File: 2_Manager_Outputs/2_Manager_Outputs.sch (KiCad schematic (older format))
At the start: 17 parts, among them J11 I2C, J2 RS232, P2 CONN_01X04, P3 SPI, P4 CONN_01X04, U1 ATMEGA328P-AU_MIO, U4 LD1117S33TR_MIO

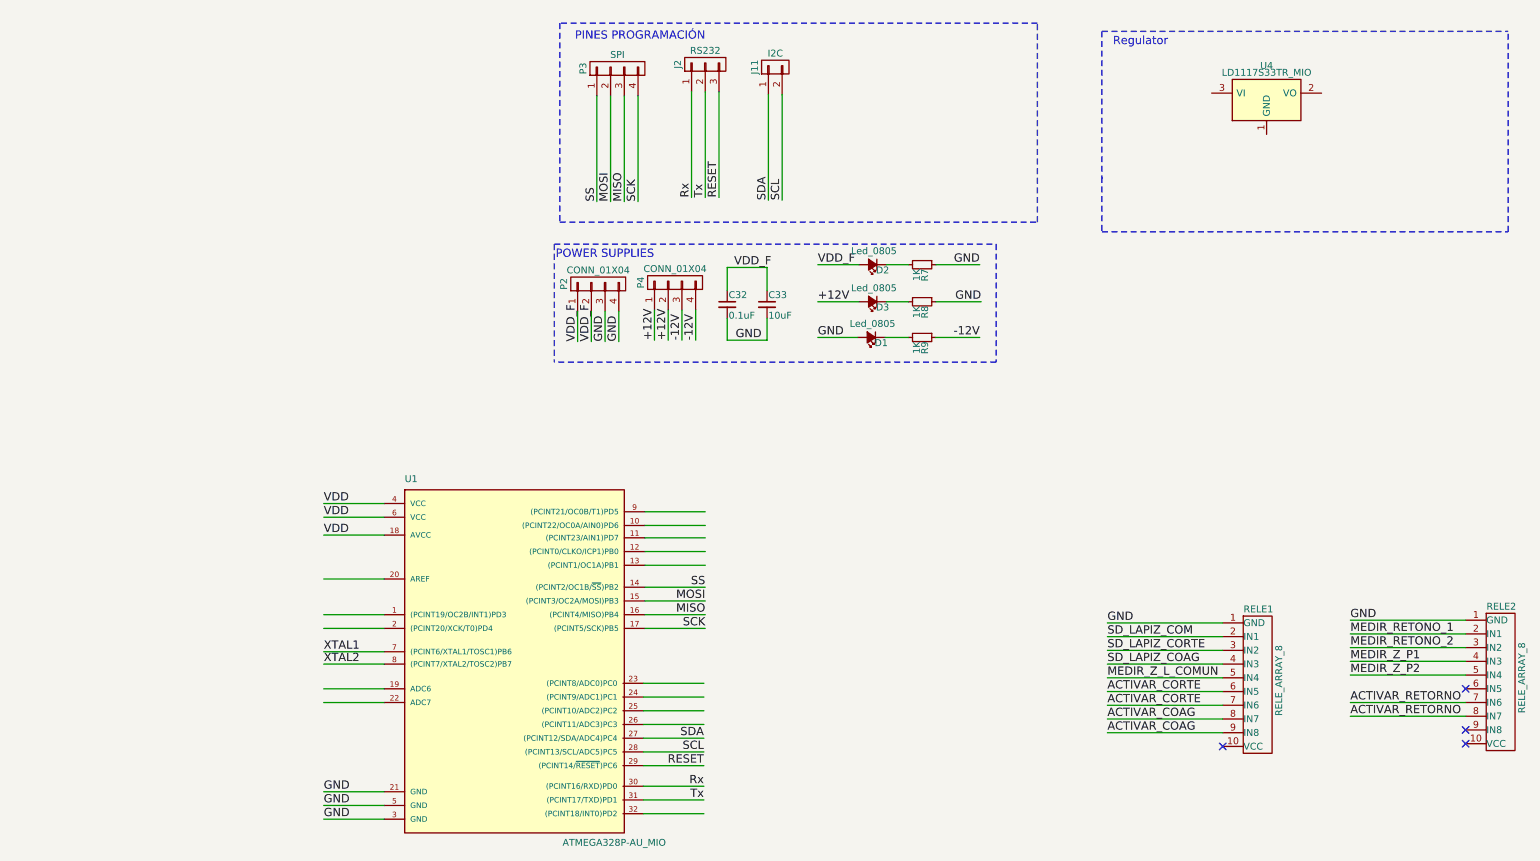
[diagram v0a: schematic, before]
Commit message: //
//
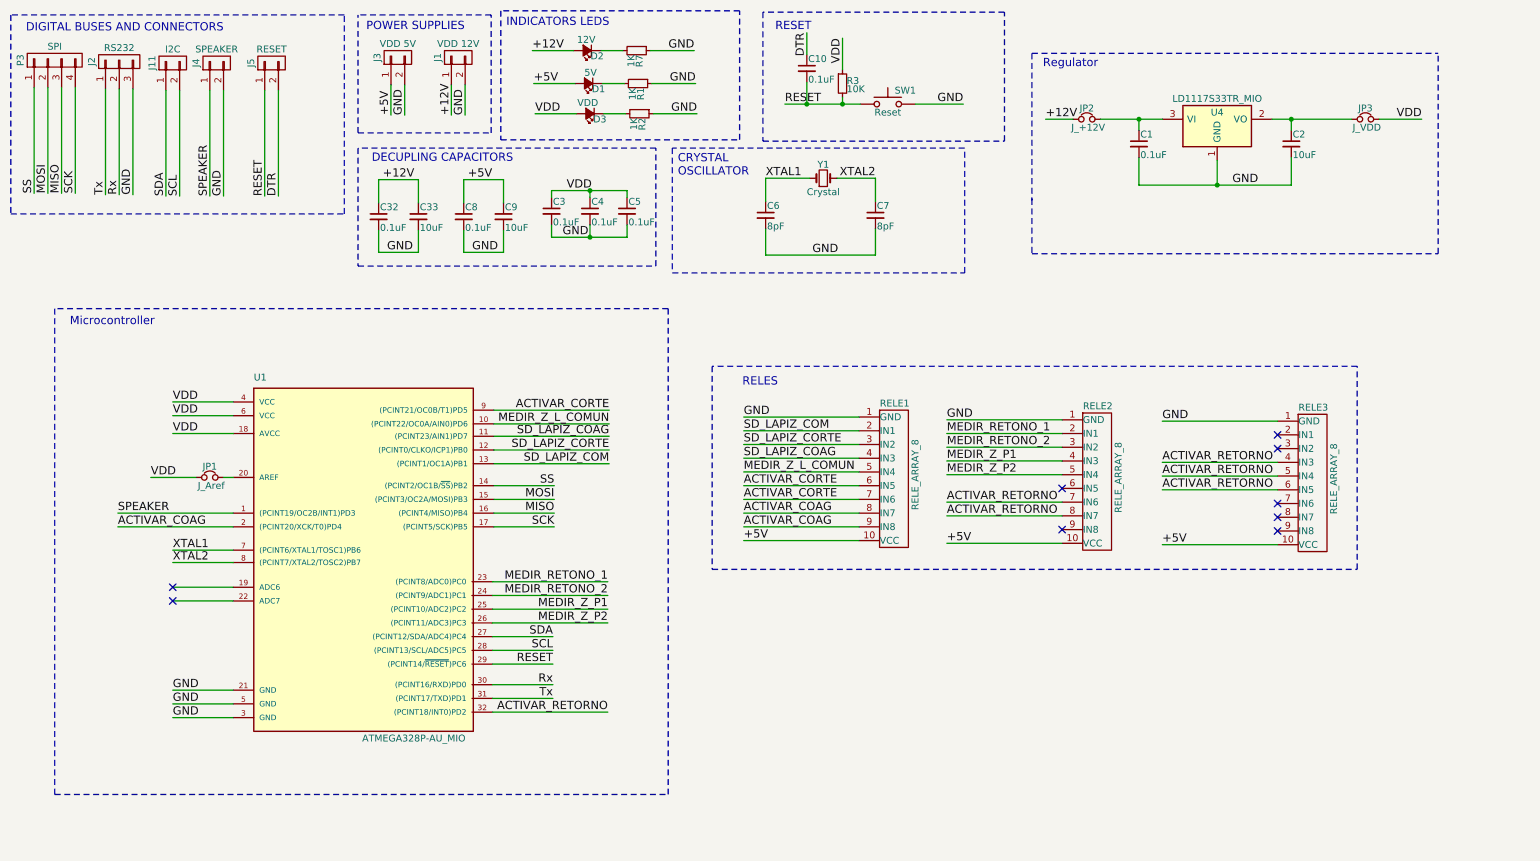
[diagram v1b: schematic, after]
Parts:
- removed P2, P4: CONN_01X04, Socket_Strips:Socket_Strip_Straight_1x04, symbol CONN_01X04
- removed R8, R9: 1K, Resistors_SMD:R_0805_HandSoldering, symbol 1K
- added C1, C10, C3, C4, C5: 0.1uF, Resistors_SMD:R_0805_HandSoldering, symbol 0.1uF
- added C2: 10uF, Resistors_SMD:R_0805_HandSoldering, symbol 10uF
- added C6, C7: 8pF, Resistors_SMD:R_0805_HandSoldering, symbol 20pF
- added C8: 0.1uF, Capacitors_SMD:C_0805_HandSoldering, symbol 0.1uF
- added C9: 10uF, Capacitors_SMD:C_0805_HandSoldering, symbol 10uF
- added J1: VDD 12V, Foot_Prints_Manager_Outputs:SUPPLY_12V, symbol CONN_01X02
- added J3: VDD 5V, Foot_Prints_Manager_Outputs:SUPPLY_5V, symbol CONN_01X02
- added J4: SPEAKER, Socket_Strips:Socket_Strip_Straight_1x02, symbol CONN_01X02
- added J5: RESET, Foot_Prints_Manager_Outputs:RESET_CONNECTOR, symbol CONN_01X02
- added JP1: J_Aref, Resistors_SMD:R_0805_HandSoldering, symbol Jumper_NC_Small
- added JP2: J_+12V, Socket_Strips:Socket_Strip_Straight_1x02, symbol Jumper_NC_Small
- added JP3: J_VDD, Socket_Strips:Socket_Strip_Straight_1x02, symbol Jumper_NC_Small
- added R1, R2: 1K, Resistors_SMD:R_0805_HandSoldering, symbol 1K
- added R3: 10K, Resistors_SMD:R_0805_HandSoldering, symbol 10K
- added RELE3: RELE_ARRAY_8, Foot_Prints_Manager_Outputs:Socket_Strip_Straight_2x10_Mio_2, symbol RELE_ARRAY_8
- added SW1: Reset, Huellas:KPT_1187B, symbol SW_Push
- added Y1: Crystal, Huellas:Crystal_SMD_XRCHA_Murata_Serie_W2,5mm_L2,0mm, symbol Crystal_Small
- D1: value Led_0805 -> 5V
- D2: value Led_0805 -> 12V
- D3: value Led_0805 -> VDD
- J11: footprint Pin_Headers:Pin_Header_Straight_1x02 -> Foot_Prints_Manager_Outputs:I2C_2X4
- J2: footprint Pin_Headers:Pin_Header_Straight_1x03 -> Foot_Prints_Manager_Outputs:RS232
- P3: footprint Socket_Strips:Socket_Strip_Straight_1x04 -> Foot_Prints_Manager_Outputs:SPI_CONNECTOR
- RELE1: footprint Socket_Strips:Socket_Strip_Angled_1x10 -> Foot_Prints_Manager_Outputs:Socket_Strip_Straight_2x10_Mio_2
- RELE2: footprint Socket_Strips:Socket_Strip_Angled_1x10 -> Foot_Prints_Manager_Outputs:Socket_Strip_Straight_2x10_Mio
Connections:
- net labels added: +5V, DTR, SPEAKER
- net labels removed: -12V, VDD_F
- wire segments 80 -> 125
- no-connect marks 4 -> 9
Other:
- note added: "CRYSTAL \nOSCILLATOR"
- note added: "DECUPLING CAPACITORS"
- note added: "DIGITAL BUSES AND CONNECTORS"
- note added: "INDICATORS LEDS"
- note added: "Microcontroller"
- note added: "RELES"
- note added: "RESET"
- note removed: "PINES PROGRAMACIÓN"
- moved on the sheet: C32, C33, D2, J11, J2, P3, R7, RELE1, RELE2, U1, U4
